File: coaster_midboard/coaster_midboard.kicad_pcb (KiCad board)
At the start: 2 copper layers, 93 x 93 mm, 6 parts, among them J1 MP, J2 MP, J3 MP, J4 MP, J5 Solderpad, J6 Solderpad

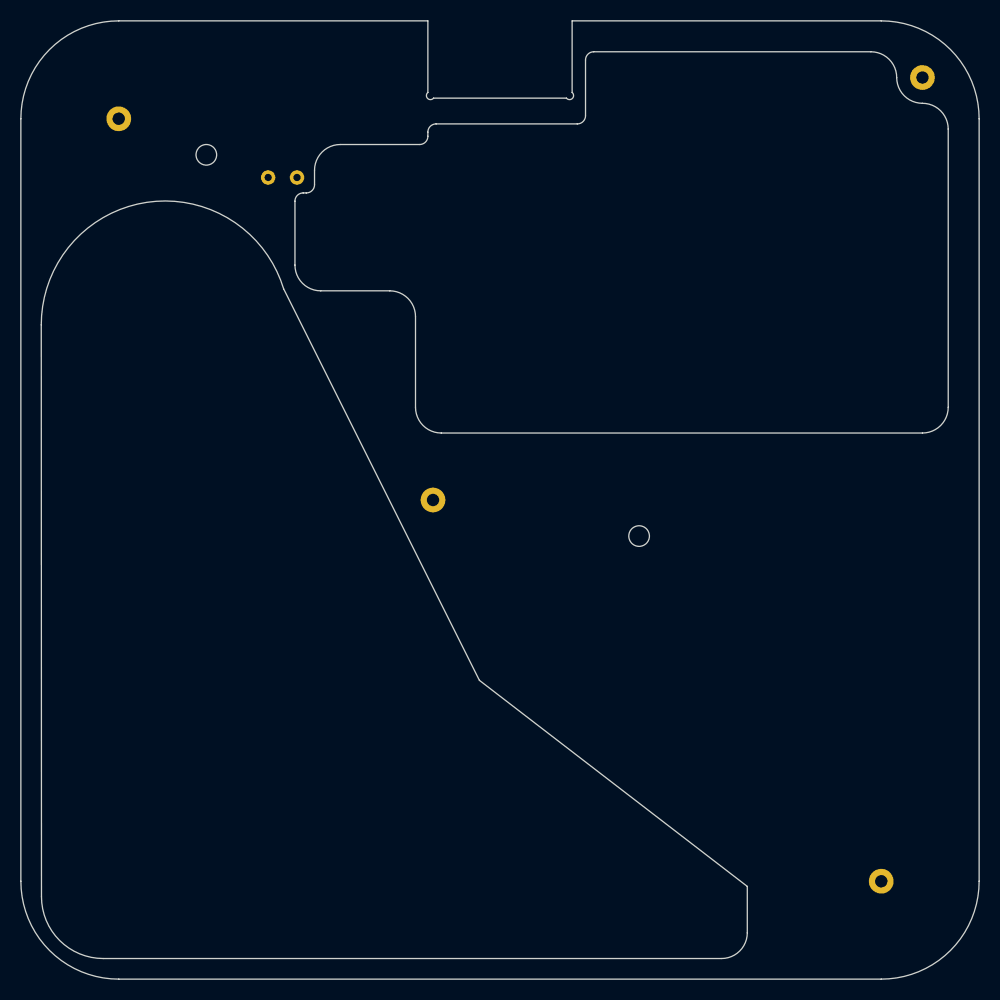
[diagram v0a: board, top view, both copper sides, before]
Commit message: updated midboard
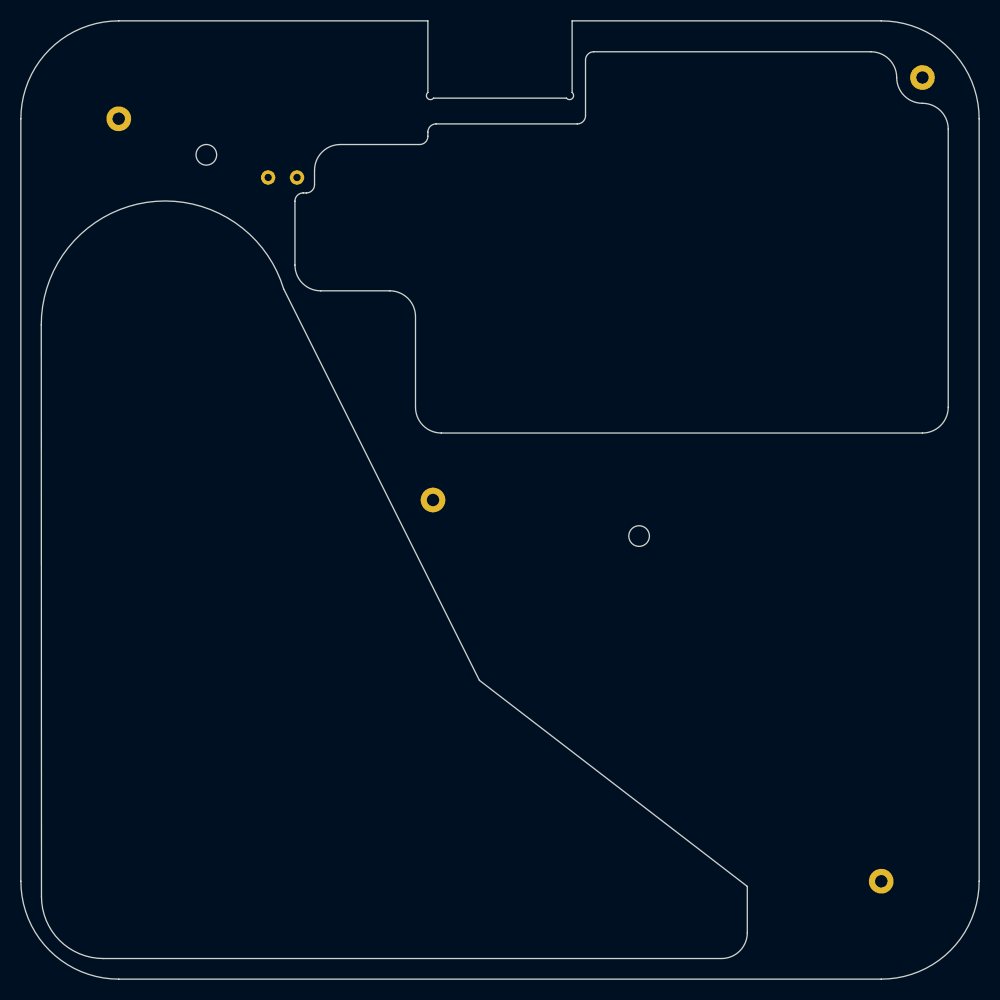
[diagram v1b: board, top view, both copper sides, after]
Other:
- net class Default removed
